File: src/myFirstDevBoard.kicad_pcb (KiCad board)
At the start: 2 copper layers, 96.5 x 68.6 mm, 36 parts, among them J1 Conn_01x15_Male, J2 Conn_01x15_Male, Q1 BC550, Q2 BC550, Q3 BC550, SW1 SW_Push, SW2 SW_Push, SW3 SW_Push, SW4 SW_Push, SW5 SW_SLIDER, SW6 SW_SLIDER

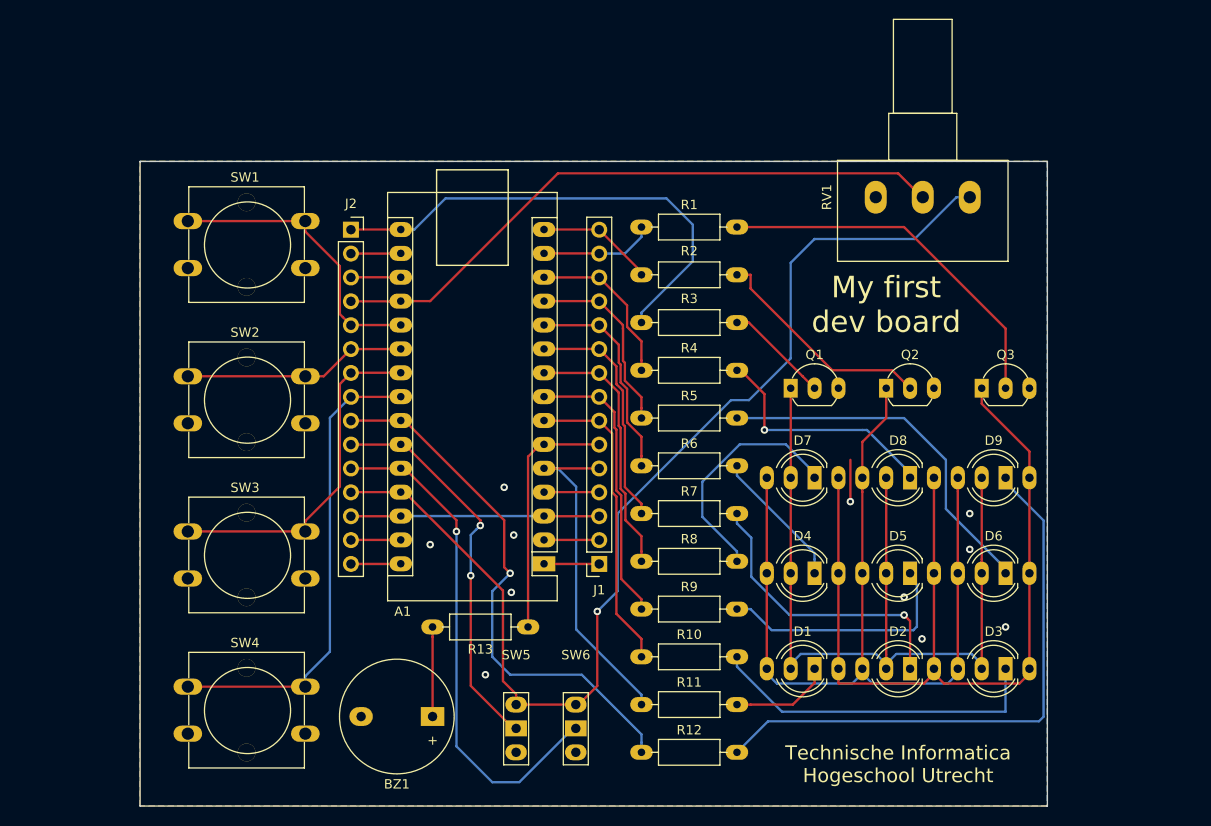
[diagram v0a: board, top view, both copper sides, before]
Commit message: adding link and rubber feet fixing #4 fixing #2
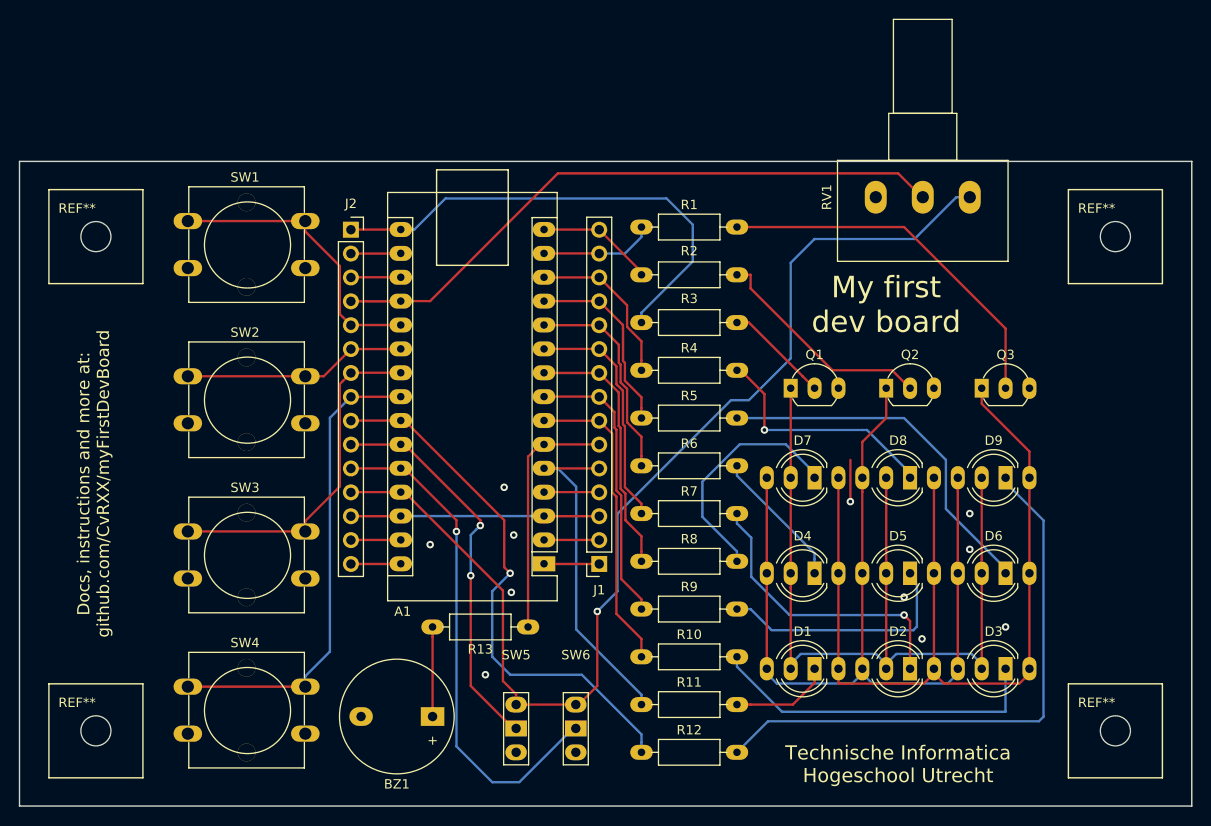
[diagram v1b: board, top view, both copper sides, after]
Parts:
- added REF**: MountingHole_3.2mm_M3_rubber_foot, lib:MountingHole_3.2mm_M3_rubber_foot, F.Cu at (109.5, 12.4)
- added REF**: MountingHole_3.2mm_M3_rubber_foot, lib:MountingHole_3.2mm_M3_rubber_foot, F.Cu at (109.5, 65.0)
- added REF**: MountingHole_3.2mm_M3_rubber_foot, lib:MountingHole_3.2mm_M3_rubber_foot, F.Cu at (1.02, 12.4)
- added REF**: MountingHole_3.2mm_M3_rubber_foot, lib:MountingHole_3.2mm_M3_rubber_foot, F.Cu at (1.02, 65.0)
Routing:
- removed copper zone on B.Cu, net GND
- removed copper zone on F.Cu, net GND
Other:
- board size 96.5 x 68.6 mm -> 124.7 x 68.6 mm
- board text added: "Docs, instructions and more at: github.com/CvRXX/myFirstDevBoard"
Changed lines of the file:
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@@
   (general
     (thickness 1.6)
-    (drawings 8)
+    (drawings 9)
     (tracks 353)
     (zones 0)
-    (modules 36)
+    (modules 40)
     (nets 45)
   )
@@
     (add_net "Net-(Q3-Pad2)")
   )
+  (module lib:MountingHole_3.2mm_M3_rubber_foot (layer F.Cu)
+    (at 109.474 12.446)
+    (descr "Mounting Hole 3.2mm, no annular, M3")
+    (tags "mounting hole 3.2mm no annular m3")
+    (attr virtual)
+    (fp_text reference REF** (at -2 -3) (layer F.SilkS)
+      (effects (font (size 1 1) (thickness 0.15)))
+    )
+    (fp_text value MountingHole_3.2mm_M3_rubber_foot (at 0 4.2) (layer F.Fab)
+      (effects (font (size 1 1) (thickness 0.15)))
+    )
+    (fp_line (start -7 7) (end -7 -7) (layer F.CrtYd) (width 0.12))
+    (fp_line (start 7 7) (end -7 7) (layer F.CrtYd) (width 0.12))
+    (fp_line (start 7 -7) (end 7 7) (layer F.CrtYd) (width 0.12))
+    (fp_line (start -7 -7) (end 7 -7) (layer F.CrtYd) (width 0.12))
+    (fp_line (start -5 5) (end -5 -5) (layer F.SilkS) (width 0.15))
+    (fp_line (start 5 5) (end -5 5) (layer F.SilkS) (width 0.15))
+    (fp_line (start 5 -5) (end 5 5) (layer F.SilkS) (width 0.15))
+    (fp_line (start -5 -5) (end 5 -5) (layer F.SilkS) (width 0.15))
+    (fp_circle (center 0 0) (end 3.2 0) (layer Cmts.User) (width 0.15))
+    (fp_text user %R (at 0.3 0) (layer F.Fab)
+      (effects (font (size 1 1) (thickness 0.15)))
+    )
+    (pad 1 np_thru_hole circle (at 0 0) (size 3.2 3.2) (drill 3.2) (layers *.Cu *.Mask))
+  )
+  (module lib:MountingHole_3.2mm_M3_rubber_foot (layer F.Cu)
+    (at 109.474 65.024)
+    (descr "Mounting Hole 3.2mm, no annular, M3")
+    (tags "mounting hole 3.2mm no annular m3")
+    (attr virtual)
+    (fp_text reference REF** (at -2 -3) (layer F.SilkS)
+      (effects (font (size 1 1) (thickness 0.15)))
+    )
+    (fp_text value MountingHole_3.2mm_M3_rubber_foot (at 0 4.2) (layer F.Fab)
+      (effects (font (size 1 1) (thickness 0.15)))
+    )
+    (fp_text user %R (at 0.3 0) (layer F.Fab)
+      (effects (font (size 1 1) (thickness 0.15)))
+    )
+    (fp_circle (center 0 0) (end 3.2 0) (layer Cmts.User) (width 0.15))
+    (fp_line (start -5 -5) (end 5 -5) (layer F.SilkS) (width 0.15))
+    (fp_line (start 5 -5) (end 5 5) (layer F.SilkS) (width 0.15))
+    (fp_line (start 5 5) (end -5 5) (layer F.SilkS) (width 0.15))
+    (fp_line (start -5 5) (end -5 -5) (layer F.SilkS) (width 0.15))
+    (fp_line (start -7 -7) (end 7 -7) (layer F.CrtYd) (width 0.12))
+    (fp_line (start 7 -7) (end 7 7) (layer F.CrtYd) (width 0.12))
+    (fp_line (start 7 7) (end -7 7) (layer F.CrtYd) (width 0.12))
+    (fp_line (start -7 7) (end -7 -7) (layer F.CrtYd) (width 0.12))
+    (pad 1 np_thru_hole circle (at 0 0) (size 3.2 3.2) (drill 3.2) (layers *.Cu *.Mask))
+  )
+  (module lib:MountingHole_3.2mm_M3_rubber_foot (layer F.Cu)
+    (at 1.016 12.446)
+    (descr "Mounting Hole 3.2mm, no annular, M3")
+    (tags "mounting hole 3.2mm no annular m3")
+    (attr virtual)
+    (fp_text reference REF** (at -2 -3) (layer F.SilkS)
+      (effects (font (size 1 1) (thickness 0.15)))
+    )
+    (fp_text value MountingHole_3.2mm_M3_rubber_foot (at 0 4.2) (layer F.Fab)
+      (effects (font (size 1 1) (thickness 0.15)))
+    )
+    (fp_text user %R (at 0.3 0) (layer F.Fab)
+      (effects (font (size 1 1) (thickness 0.15)))
+    )
+    (fp_circle (center 0 0) (end 3.2 0) (layer Cmts.User) (width 0.15))
+    (fp_line (start -5 -5) (end 5 -5) (layer F.SilkS) (width 0.15))
+    (fp_line (start 5 -5) (end 5 5) (layer F.SilkS) (width 0.15))
+    (fp_line (start 5 5) (end -5 5) (layer F.SilkS) (width 0.15))
+    (fp_line (start -5 5) (end -5 -5) (layer F.SilkS) (width 0.15))
+    (fp_line (start -7 -7) (end 7 -7) (layer F.CrtYd) (width 0.12))
+    (fp_line (start 7 -7) (end 7 7) (layer F.CrtYd) (width 0.12))
+    (fp_line (start 7 7) (end -7 7) (layer F.CrtYd) (width 0.12))
+    (fp_line (start -7 7) (end -7 -7) (layer F.CrtYd) (width 0.12))
+    (pad 1 np_thru_hole circle (at 0 0) (size 3.2 3.2) (drill 3.2) (layers *.Cu *.Mask))
+  )
+  (module lib:MountingHole_3.2mm_M3_rubber_foot (layer F.Cu)
+    (at 1.016 65.024)
+    (descr "Mounting Hole 3.2mm, no annular, M3")
+    (tags "mounting hole 3.2mm no annular m3")
+    (attr virtual)
+    (fp_text reference REF** (at -2 -3) (layer F.SilkS)
+      (effects (font (size 1 1) (thickness 0.15)))
+    )
+    (fp_text value MountingHole_3.2mm_M3_rubber_foot (at 0 4.2) (layer F.Fab)
+      (effects (font (size 1 1) (thickness 0.15)))
+    )
+    (fp_line (start -7 7) (end -7 -7) (layer F.CrtYd) (width 0.12))
+    (fp_line (start 7 7) (end -7 7) (layer F.CrtYd) (width 0.12))
+    (fp_line (start 7 -7) (end 7 7) (layer F.CrtYd) (width 0.12))
+    (fp_line (start -7 -7) (end 7 -7) (layer F.CrtYd) (width 0.12))
+    (fp_line (start -5 5) (end -5 -5) (layer F.SilkS) (width 0.15))
+    (fp_line (start 5 5) (end -5 5) (layer F.SilkS) (width 0.15))
+    (fp_line (start 5 -5) (end 5 5) (layer F.SilkS) (width 0.15))
+    (fp_line (start -5 -5) (end 5 -5) (layer F.SilkS) (width 0.15))
+    (fp_circle (center 0 0) (end 3.2 0) (layer Cmts.User) (width 0.15))
+    (fp_text user %R (at 0.3 0) (layer F.Fab)
+      (effects (font (size 1 1) (thickness 0.15)))
+    )
+    (pad 1 np_thru_hole circle (at 0 0) (size 3.2 3.2) (drill 3.2) (layers *.Cu *.Mask))
+  )
   (module lib:LED_D5.0mm-4_RGB_wide (layer F.Cu)
     (at 84.455 38.1)
@@
     )
   )
+  (gr_text "Docs, instructions and more at:\ngithub.com/CvRXX/myFirstDevBoard" (at 0.762 38.735 90) (layer F.SilkS)
+    (effects (font (size 1.3 1.3) (thickness 0.3)))
+  )
   (gr_text V1.00 (at 10.16 71.12) (layer B.SilkS)
     (effects (font (size 1.5 1.5) (thickness 0.3)) (justify mirror))
@@
     (effects (font (size 1.5 1.5) (thickness 0.3)) (justify mirror))
   )
-  (gr_line (start 102.235 73.025) (end 102.235 4.445) (layer Edge.Cuts) (width 0.15))
-  (gr_line (start 5.715 73.025) (end 102.235 73.025) (layer Edge.Cuts) (width 0.15))
-  (gr_line (start 5.715 4.445) (end 5.715 73.025) (layer Edge.Cuts) (width 0.15))
-  (gr_line (start 102.235 4.445) (end 5.715 4.445) (layer Edge.Cuts) (width 0.15))
+  (gr_line (start 117.602 73.025) (end 117.602 4.445) (layer Edge.Cuts) (width 0.15))
+  (gr_line (start -7.112 73.025) (end 117.602 73.025) (layer Edge.Cuts) (width 0.15))
+  (gr_line (start -7.112 4.445) (end -7.112 73.025) (layer Edge.Cuts) (width 0.15))
+  (gr_line (start 117.602 4.445) (end -7.112 4.445) (layer Edge.Cuts) (width 0.15))
   (segment (start 48.709553 47.272379) (end 48.688552 47.251378) (width 0.25) (layer F.Cu) (net 1))
   (segment (start 54.561553 47.272379) (end 48.709553 47.272379) (width 0.25) (layer F.Cu) (net 1))
@@
   (segment (start 101.346 64.008) (end 72.517 64.008) (width 0.25) (layer B.Cu) (net 44))
   (segment (start 97.79 38.6) (end 101.83499 42.64499) (width 0.25) (layer B.Cu) (net 44))
-  (zone (net 6) (net_name GND) (layer F.Cu) (hatch edge 0.508)
-    (connect_pads (clearance 0.508))
-    (min_thickness 0.254)
-    (fill yes (arc_segments 16) (thermal_gap 0.508) (thermal_bridge_width 0.508))
-    (polygon
-      (pts
-        (xy 5.715 4.445) (xy 102.235 4.445) (xy 102.235 73.025) (xy 5.715 73.025)
-      )
-    )
-  )
-  (zone (net 6) (net_name GND) (layer B.Cu) (hatch edge 0.508)
-    (connect_pads (clearance 0.508))
-    (min_thickness 0.254)
-    (fill yes (arc_segments 16) (thermal_gap 0.508) (thermal_bridge_width 0.508))
-    (polygon
-      (pts
-        (xy 102.235 4.445) (xy 102.235 73.025) (xy 5.715 73.025) (xy 5.715 4.445)
-      )
-    )
-  )
 )

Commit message: Revert "adding link and rubber feet" This is reverted because the board is now to big for fab
This reverts commit 696723d42228766d8a1a20b6e9d58cdf75adf79a.
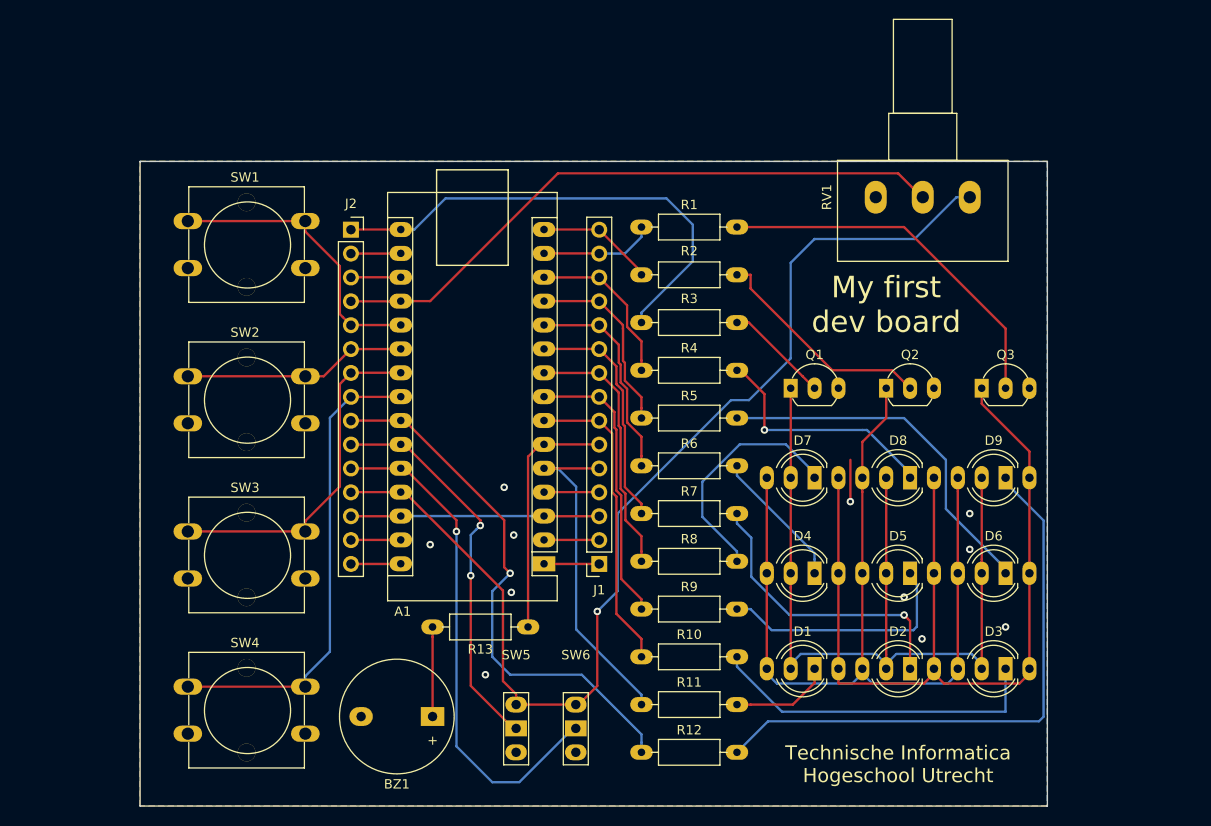
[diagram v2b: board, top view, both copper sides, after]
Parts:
- removed REF** (x4): MountingHole_3.2mm_M3_rubber_foot, lib:MountingHole_3.2mm_M3_rubber_foot
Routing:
- added copper zone on B.Cu, net GND
- added copper zone on F.Cu, net GND
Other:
- board size 124.7 x 68.6 mm -> 96.5 x 68.6 mm
- board text removed: "Docs, instructions and more at: github.com/CvRXX/myFirstDevBoard"
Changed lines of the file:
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@@
   (general
     (thickness 1.6)
-    (drawings 9)
+    (drawings 8)
     (tracks 353)
     (zones 0)
-    (modules 40)
+    (modules 36)
     (nets 45)
   )
@@
     (add_net "Net-(Q3-Pad2)")
   )
-  (module lib:MountingHole_3.2mm_M3_rubber_foot (layer F.Cu)
-    (at 109.474 12.446)
-    (descr "Mounting Hole 3.2mm, no annular, M3")
-    (tags "mounting hole 3.2mm no annular m3")
-    (attr virtual)
-    (fp_text reference REF** (at -2 -3) (layer F.SilkS)
-      (effects (font (size 1 1) (thickness 0.15)))
-    )
-    (fp_text value MountingHole_3.2mm_M3_rubber_foot (at 0 4.2) (layer F.Fab)
-      (effects (font (size 1 1) (thickness 0.15)))
-    )
-    (fp_line (start -7 7) (end -7 -7) (layer F.CrtYd) (width 0.12))
-    (fp_line (start 7 7) (end -7 7) (layer F.CrtYd) (width 0.12))
-    (fp_line (start 7 -7) (end 7 7) (layer F.CrtYd) (width 0.12))
-    (fp_line (start -7 -7) (end 7 -7) (layer F.CrtYd) (width 0.12))
-    (fp_line (start -5 5) (end -5 -5) (layer F.SilkS) (width 0.15))
-    (fp_line (start 5 5) (end -5 5) (layer F.SilkS) (width 0.15))
-    (fp_line (start 5 -5) (end 5 5) (layer F.SilkS) (width 0.15))
-    (fp_line (start -5 -5) (end 5 -5) (layer F.SilkS) (width 0.15))
-    (fp_circle (center 0 0) (end 3.2 0) (layer Cmts.User) (width 0.15))
-    (fp_text user %R (at 0.3 0) (layer F.Fab)
-      (effects (font (size 1 1) (thickness 0.15)))
-    )
-    (pad 1 np_thru_hole circle (at 0 0) (size 3.2 3.2) (drill 3.2) (layers *.Cu *.Mask))
-  )
-  (module lib:MountingHole_3.2mm_M3_rubber_foot (layer F.Cu)
-    (at 109.474 65.024)
-    (descr "Mounting Hole 3.2mm, no annular, M3")
-    (tags "mounting hole 3.2mm no annular m3")
-    (attr virtual)
-    (fp_text reference REF** (at -2 -3) (layer F.SilkS)
-      (effects (font (size 1 1) (thickness 0.15)))
-    )
-    (fp_text value MountingHole_3.2mm_M3_rubber_foot (at 0 4.2) (layer F.Fab)
-      (effects (font (size 1 1) (thickness 0.15)))
-    )
-    (fp_text user %R (at 0.3 0) (layer F.Fab)
-      (effects (font (size 1 1) (thickness 0.15)))
-    )
-    (fp_circle (center 0 0) (end 3.2 0) (layer Cmts.User) (width 0.15))
-    (fp_line (start -5 -5) (end 5 -5) (layer F.SilkS) (width 0.15))
-    (fp_line (start 5 -5) (end 5 5) (layer F.SilkS) (width 0.15))
-    (fp_line (start 5 5) (end -5 5) (layer F.SilkS) (width 0.15))
-    (fp_line (start -5 5) (end -5 -5) (layer F.SilkS) (width 0.15))
-    (fp_line (start -7 -7) (end 7 -7) (layer F.CrtYd) (width 0.12))
-    (fp_line (start 7 -7) (end 7 7) (layer F.CrtYd) (width 0.12))
-    (fp_line (start 7 7) (end -7 7) (layer F.CrtYd) (width 0.12))
-    (fp_line (start -7 7) (end -7 -7) (layer F.CrtYd) (width 0.12))
-    (pad 1 np_thru_hole circle (at 0 0) (size 3.2 3.2) (drill 3.2) (layers *.Cu *.Mask))
-  )
-  (module lib:MountingHole_3.2mm_M3_rubber_foot (layer F.Cu)
-    (at 1.016 12.446)
-    (descr "Mounting Hole 3.2mm, no annular, M3")
-    (tags "mounting hole 3.2mm no annular m3")
-    (attr virtual)
-    (fp_text reference REF** (at -2 -3) (layer F.SilkS)
-      (effects (font (size 1 1) (thickness 0.15)))
-    )
-    (fp_text value MountingHole_3.2mm_M3_rubber_foot (at 0 4.2) (layer F.Fab)
-      (effects (font (size 1 1) (thickness 0.15)))
-    )
-    (fp_text user %R (at 0.3 0) (layer F.Fab)
-      (effects (font (size 1 1) (thickness 0.15)))
-    )
-    (fp_circle (center 0 0) (end 3.2 0) (layer Cmts.User) (width 0.15))
-    (fp_line (start -5 -5) (end 5 -5) (layer F.SilkS) (width 0.15))
-    (fp_line (start 5 -5) (end 5 5) (layer F.SilkS) (width 0.15))
-    (fp_line (start 5 5) (end -5 5) (layer F.SilkS) (width 0.15))
-    (fp_line (start -5 5) (end -5 -5) (layer F.SilkS) (width 0.15))
-    (fp_line (start -7 -7) (end 7 -7) (layer F.CrtYd) (width 0.12))
-    (fp_line (start 7 -7) (end 7 7) (layer F.CrtYd) (width 0.12))
-    (fp_line (start 7 7) (end -7 7) (layer F.CrtYd) (width 0.12))
-    (fp_line (start -7 7) (end -7 -7) (layer F.CrtYd) (width 0.12))
-    (pad 1 np_thru_hole circle (at 0 0) (size 3.2 3.2) (drill 3.2) (layers *.Cu *.Mask))
-  )
-  (module lib:MountingHole_3.2mm_M3_rubber_foot (layer F.Cu)
-    (at 1.016 65.024)
-    (descr "Mounting Hole 3.2mm, no annular, M3")
-    (tags "mounting hole 3.2mm no annular m3")
-    (attr virtual)
-    (fp_text reference REF** (at -2 -3) (layer F.SilkS)
-      (effects (font (size 1 1) (thickness 0.15)))
-    )
-    (fp_text value MountingHole_3.2mm_M3_rubber_foot (at 0 4.2) (layer F.Fab)
-      (effects (font (size 1 1) (thickness 0.15)))
-    )
-    (fp_line (start -7 7) (end -7 -7) (layer F.CrtYd) (width 0.12))
-    (fp_line (start 7 7) (end -7 7) (layer F.CrtYd) (width 0.12))
-    (fp_line (start 7 -7) (end 7 7) (layer F.CrtYd) (width 0.12))
-    (fp_line (start -7 -7) (end 7 -7) (layer F.CrtYd) (width 0.12))
-    (fp_line (start -5 5) (end -5 -5) (layer F.SilkS) (width 0.15))
-    (fp_line (start 5 5) (end -5 5) (layer F.SilkS) (width 0.15))
-    (fp_line (start 5 -5) (end 5 5) (layer F.SilkS) (width 0.15))
-    (fp_line (start -5 -5) (end 5 -5) (layer F.SilkS) (width 0.15))
-    (fp_circle (center 0 0) (end 3.2 0) (layer Cmts.User) (width 0.15))
-    (fp_text user %R (at 0.3 0) (layer F.Fab)
-      (effects (font (size 1 1) (thickness 0.15)))
-    )
-    (pad 1 np_thru_hole circle (at 0 0) (size 3.2 3.2) (drill 3.2) (layers *.Cu *.Mask))
-  )
   (module lib:LED_D5.0mm-4_RGB_wide (layer F.Cu)
     (at 84.455 38.1)
@@
     )
   )
-  (gr_text "Docs, instructions and more at:\ngithub.com/CvRXX/myFirstDevBoard" (at 0.762 38.735 90) (layer F.SilkS)
-    (effects (font (size 1.3 1.3) (thickness 0.3)))
-  )
   (gr_text V1.00 (at 10.16 71.12) (layer B.SilkS)
     (effects (font (size 1.5 1.5) (thickness 0.3)) (justify mirror))
@@
     (effects (font (size 1.5 1.5) (thickness 0.3)) (justify mirror))
   )
-  (gr_line (start 117.602 73.025) (end 117.602 4.445) (layer Edge.Cuts) (width 0.15))
-  (gr_line (start -7.112 73.025) (end 117.602 73.025) (layer Edge.Cuts) (width 0.15))
-  (gr_line (start -7.112 4.445) (end -7.112 73.025) (layer Edge.Cuts) (width 0.15))
-  (gr_line (start 117.602 4.445) (end -7.112 4.445) (layer Edge.Cuts) (width 0.15))
+  (gr_line (start 102.235 73.025) (end 102.235 4.445) (layer Edge.Cuts) (width 0.15))
+  (gr_line (start 5.715 73.025) (end 102.235 73.025) (layer Edge.Cuts) (width 0.15))
+  (gr_line (start 5.715 4.445) (end 5.715 73.025) (layer Edge.Cuts) (width 0.15))
+  (gr_line (start 102.235 4.445) (end 5.715 4.445) (layer Edge.Cuts) (width 0.15))
   (segment (start 48.709553 47.272379) (end 48.688552 47.251378) (width 0.25) (layer F.Cu) (net 1))
   (segment (start 54.561553 47.272379) (end 48.709553 47.272379) (width 0.25) (layer F.Cu) (net 1))
@@
   (segment (start 101.346 64.008) (end 72.517 64.008) (width 0.25) (layer B.Cu) (net 44))
   (segment (start 97.79 38.6) (end 101.83499 42.64499) (width 0.25) (layer B.Cu) (net 44))
+  (zone (net 6) (net_name GND) (layer F.Cu) (hatch edge 0.508)
+    (connect_pads (clearance 0.508))
+    (min_thickness 0.254)
+    (fill yes (arc_segments 16) (thermal_gap 0.508) (thermal_bridge_width 0.508))
+    (polygon
+      (pts
+        (xy 5.715 4.445) (xy 102.235 4.445) (xy 102.235 73.025) (xy 5.715 73.025)
+      )
+    )
+  )
+  (zone (net 6) (net_name GND) (layer B.Cu) (hatch edge 0.508)
+    (connect_pads (clearance 0.508))
+    (min_thickness 0.254)
+    (fill yes (arc_segments 16) (thermal_gap 0.508) (thermal_bridge_width 0.508))
+    (polygon
+      (pts
+        (xy 102.235 4.445) (xy 102.235 73.025) (xy 5.715 73.025) (xy 5.715 4.445)
+      )
+    )
+  )
 )
